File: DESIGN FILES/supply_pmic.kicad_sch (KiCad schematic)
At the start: 24 parts, among them U5 UM805RE, U6 UM803RS

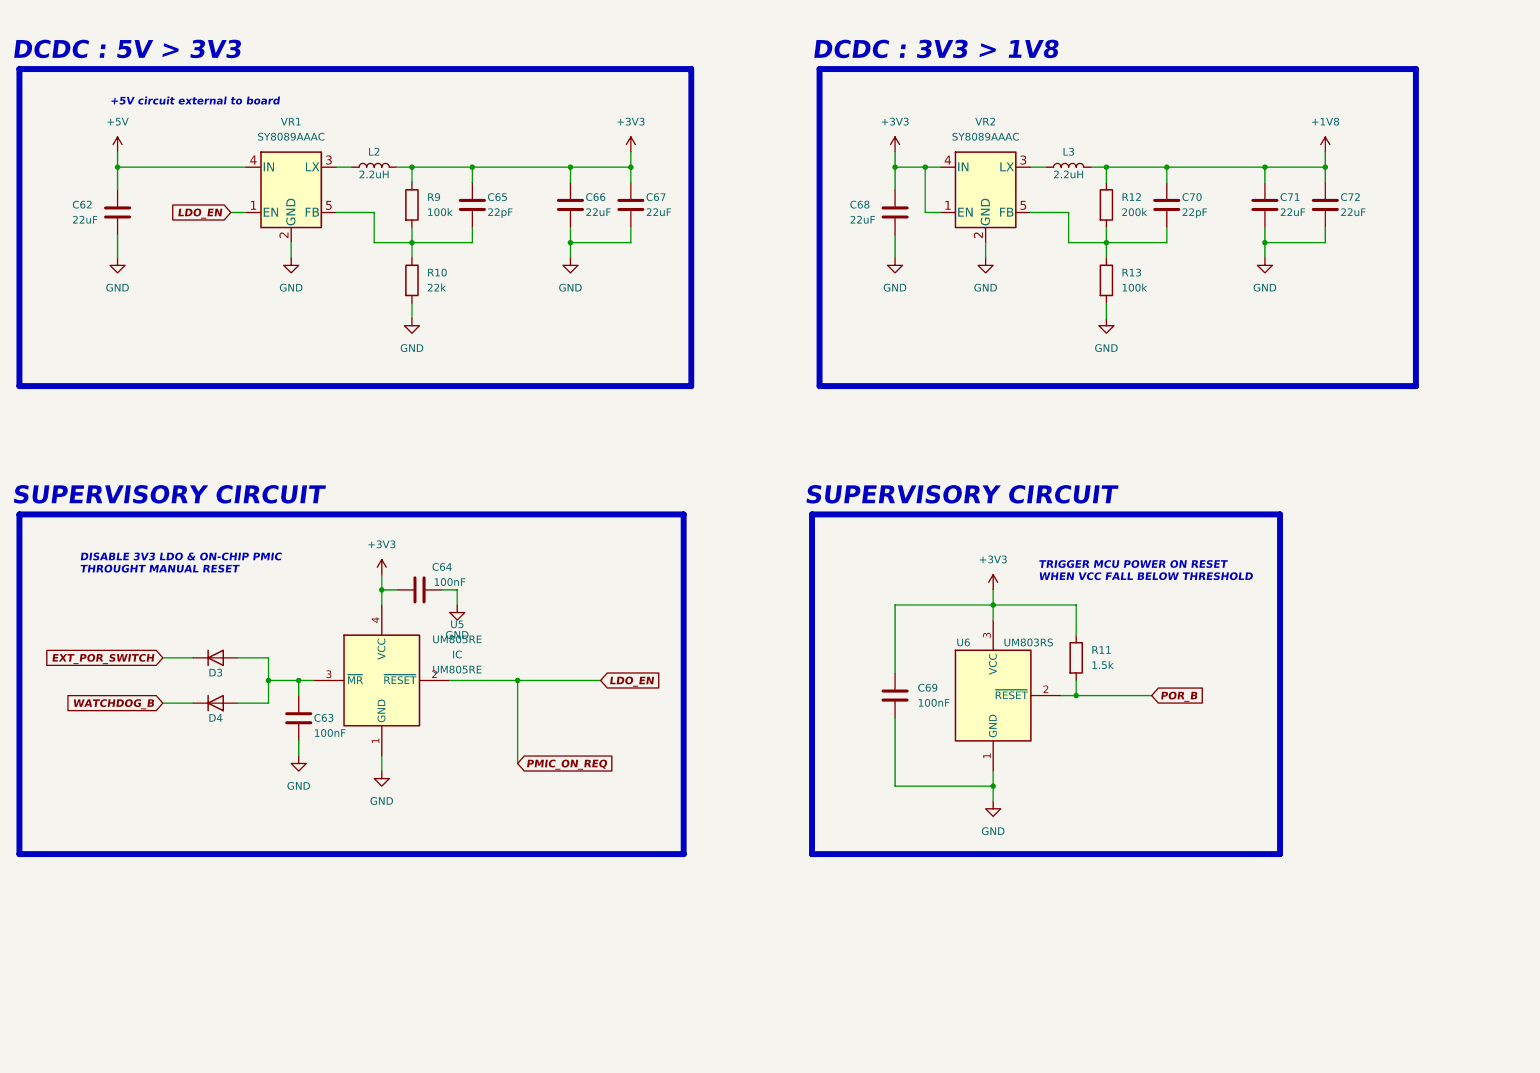
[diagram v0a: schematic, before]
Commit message: work
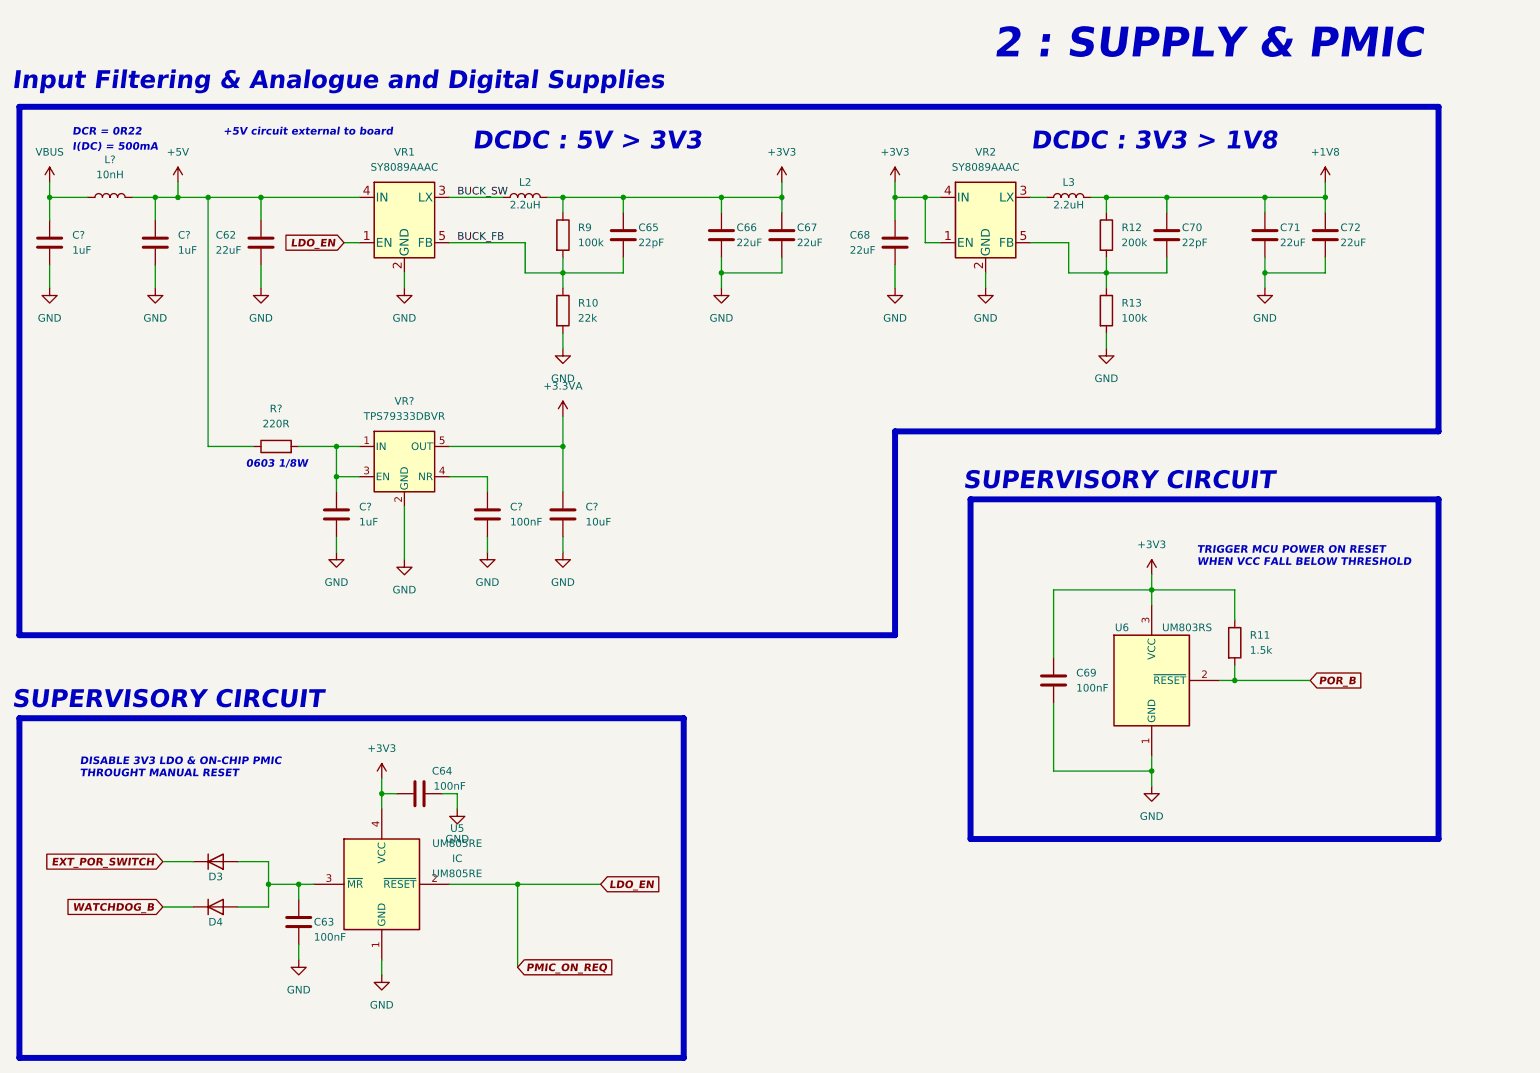
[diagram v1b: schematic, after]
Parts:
- added C?: 100nF, symbol MIMXRT1064 MCU Module:CL05B104KB54PNC
- added C? (x3): 1uF, symbol MIMXRT1064 MCU Module:CL05A105KA5NQNC
- added C?: 10uF, symbol MIMXRT1064 MCU Module:CL10A106KP8NNNC
- added L?: 10nH, symbol MIMXRT1064 MCU Module:MLG1005S10NHT000
- added R?: 220R, symbol MIMXRT1064 MCU Module:0603WAF2200T5E
- added VR?: TPS79333DBVR, Package_TO_SOT_SMD:SOT-23-5, symbol MIMXRT1064 MCU Module:TPS79333DBVR
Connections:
- net +5V: now also C?.1, L?.2, R?.1
- net GND: now also C?.2, C?.2, C?.2, C?.2, C?.2, VR?.2 (GND)
- net BUCK_FB: now reaches C65.2, R10.1, R9.2, VR1.5 (FB)
- net BUCK_SW: now reaches L2.1, VR1.3 (LX)
- new net: C?.1, VR?.4 (NR)
- new net: C?.1, R?.2, VR?.1 (IN), VR?.3 (EN)
- new net +3.3VA: C?.1, VR?.5 (OUT)
- new net VBUS: C?.1, L?.1
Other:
- note added: "0603 1/8W"
- note added: "2 : SUPPLY & PMIC"
- note added: "DCR = 0R22"
- note added: "I(DC) = 500mA"
- note added: "Input Filtering & Analogue and Digital Supplies"
- company: (none) -> Soundsom
- title: (none) -> Supply & PMIC
- moved on the sheet: C62, C63, C64, C65, C66, C67, C68, C69, C70, C71, C72, D3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
